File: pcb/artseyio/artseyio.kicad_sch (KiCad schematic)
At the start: 21 parts, among them J1 USB_C16PIN, J2 BOOT, SW1 SW_MEC_5G, SW2 SW_MEC_5G, SW3 SW_MEC_5G, SW4 SW_MEC_5G, SW5 SW_MEC_5G, SW6 SW_MEC_5G, SW7 SW_MEC_5G, SW8 SW_MEC_5G, U3 CH552G

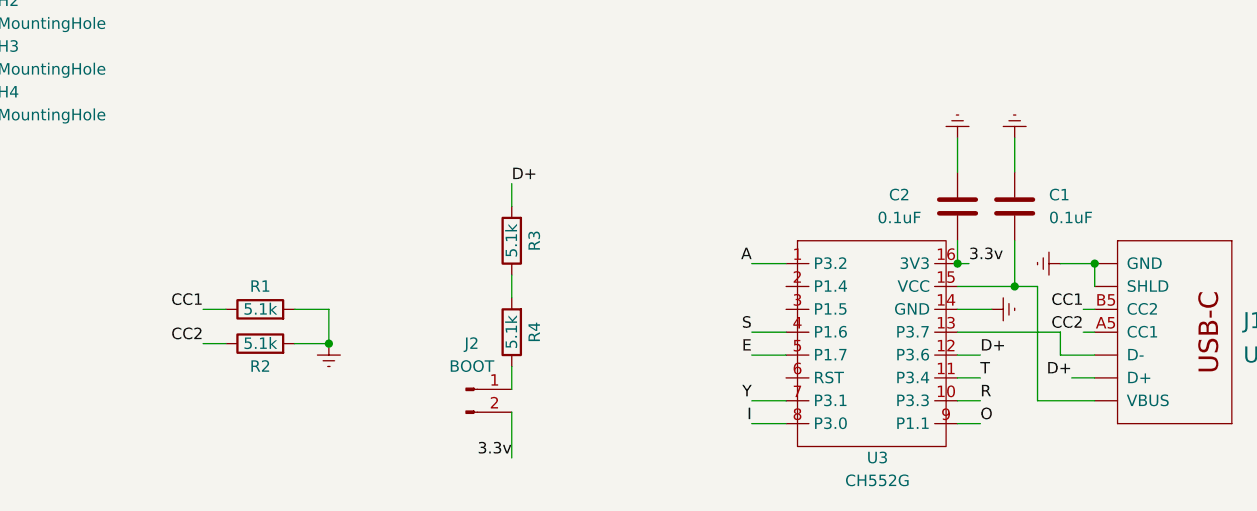
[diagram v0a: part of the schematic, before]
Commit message: Reverted PCB also.
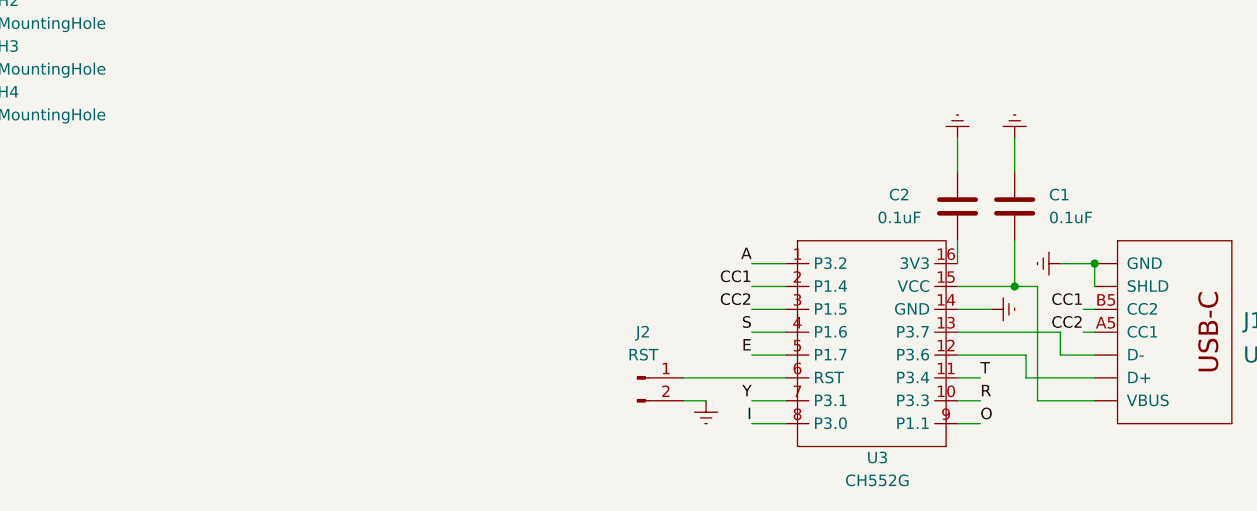
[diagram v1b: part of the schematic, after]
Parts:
- removed R1, R2, R3, R4: 5.1k, Resistor_SMD:R_0805_2012Metric, symbol Device:R
- J2: value BOOT -> RST
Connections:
- net CC1: now also U3.2 (P1.4)
- net CC2: now also U3.3 (P1.5)
- net Earth: now also J2.2 (Pin_2)
- net at J2.1 (Pin_1): now also U3.6 (RST)
- net 3.3v: no longer names the net of C2.2, U3.16 (3V3)
- net 3.3v: no longer J2.2 (Pin_2)
- net D+: no longer names the net of J1.A6 (D+), J1.B6 (D+), U3.12 (P3.6)
